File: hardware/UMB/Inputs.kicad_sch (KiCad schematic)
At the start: 30 parts, among them J1 FTSH-107-01-L-D-K, J10 Conn_01x04, J11 Conn_01x04, J12 Conn_01x04, J13 Conn_01x04, J14 Conn_01x04, J15 Conn_01x04, J2 Conn_01x02, J3 Conn_01x02, J4 Conn_01x03, J5 Conn_01x03, J6 Conn_01x03, J7 Conn_01x03, J8 Conn_01x03, J9 Conn_01x03

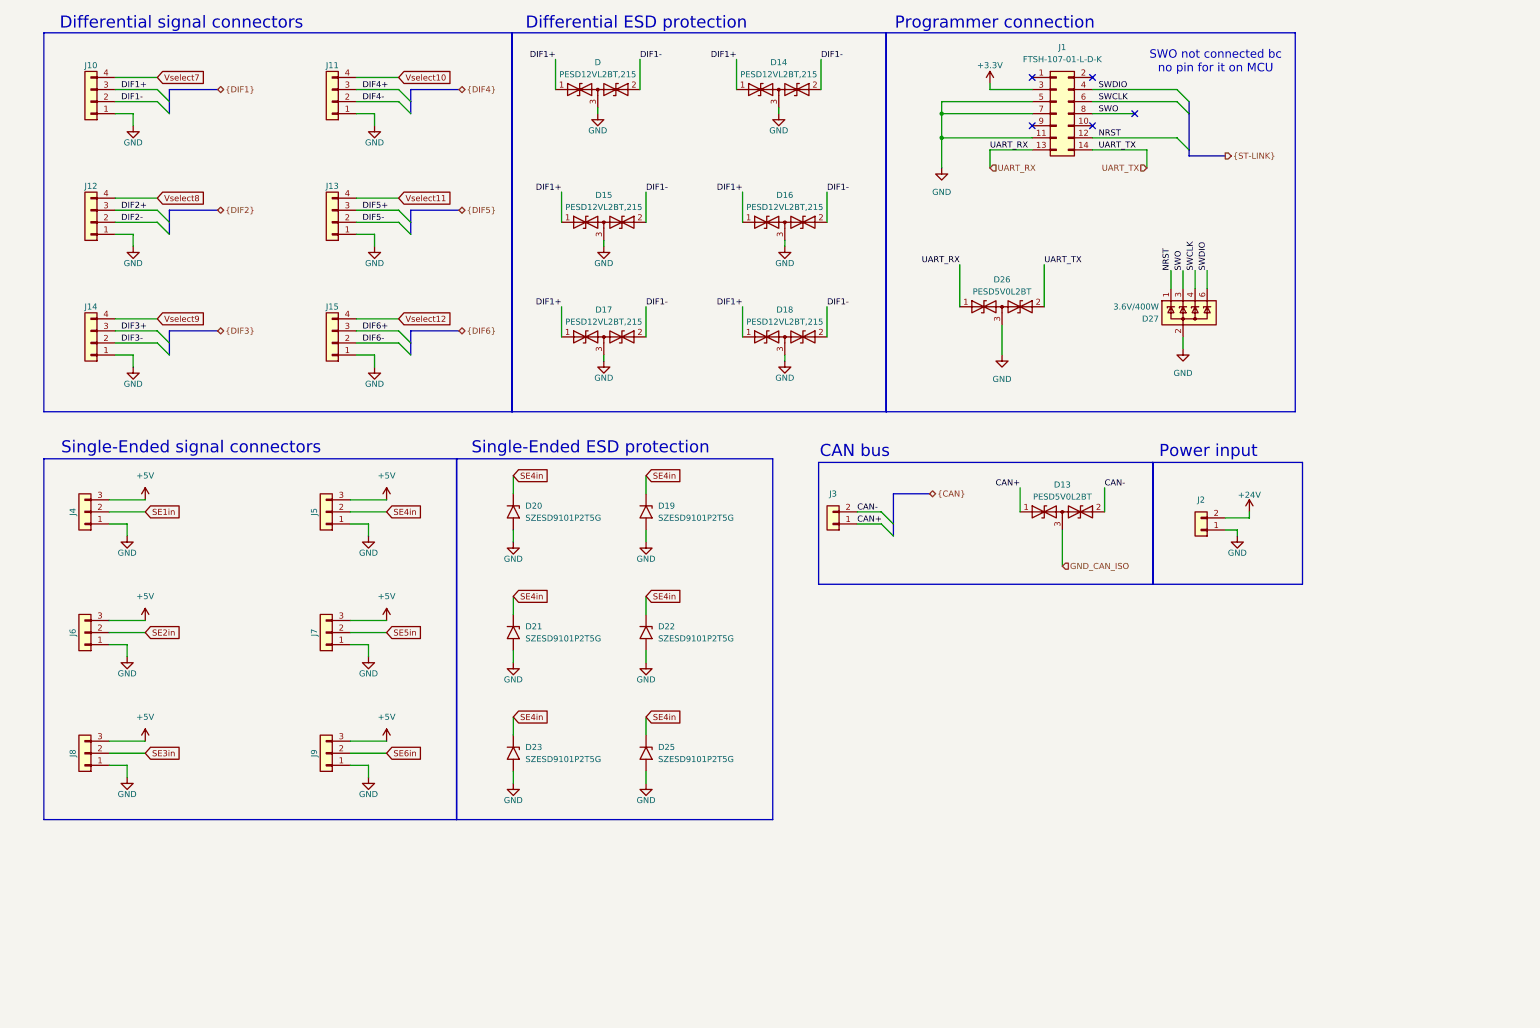
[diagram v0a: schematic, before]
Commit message: Power section done
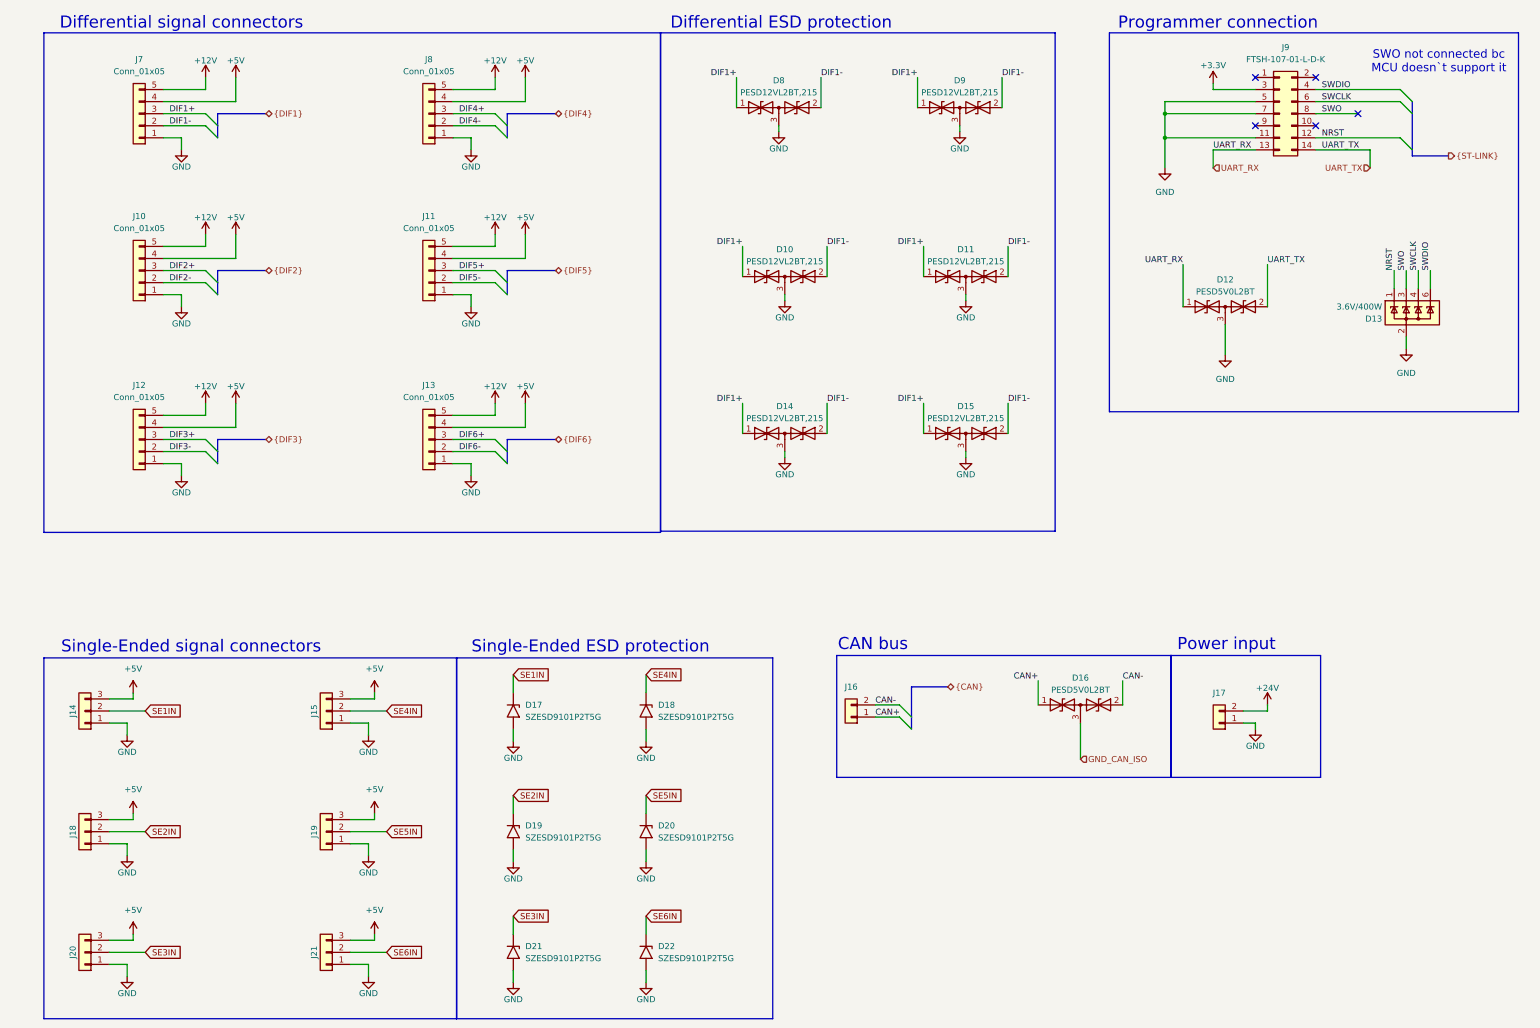
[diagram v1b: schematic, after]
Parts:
- removed J10, J11, J12, J13, J14, J15: Conn_01x04, symbol Connector_Generic:Conn_01x04
- added J10, J11, J12, J13, J7, J8: Conn_01x05, symbol Connector_Generic:Conn_01x05
- renumbered D15 to D10, D16 to D11, D26 to D12, D27 to D13, D17 to D14, D18 to D15, D13 to D16, D20 to D17, D19 to D18, D21 to D19, D22 to D20, D23 to D21, D25 to D22, D to D8, D14 to D9, J4 to J14, J5 to J15, J3 to J16, J2 to J17, J6 to J18, J7 to J19, J8 to J20, J9 to J21, J1 to J9
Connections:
- net +5V: now also J10.4 (Pin_4), J11.4 (Pin_4), J12.4 (Pin_4), J13.4 (Pin_4), J7.4 (Pin_4), J8.4 (Pin_4)
- net DIF1+: now also J7.3 (Pin_3)
- net DIF1-: now also J7.2 (Pin_2)
- net DIF2+: now also J10.3 (Pin_3)
- net DIF2-: now also J10.2 (Pin_2)
- net DIF3+: now also J12.3 (Pin_3)
- net DIF3-: now also J12.2 (Pin_2)
- net DIF4+: now also J8.3 (Pin_3)
- net DIF4-: now also J8.2 (Pin_2)
- net DIF5+: now also J11.3 (Pin_3)
- net DIF5-: now also J11.2 (Pin_2)
- net DIF6+: now also J13.3 (Pin_3)
- net DIF6-: now also J13.2 (Pin_2)
- net GND: now also J10.1 (Pin_1), J11.1 (Pin_1), J12.1 (Pin_1), J13.1 (Pin_1), J7.1 (Pin_1), J8.1 (Pin_1)
- net SE1in renamed SE1IN
- net SE1IN: now also D17.1 (A1)
- net SE2in renamed SE2IN
- net SE2IN: now also D19.1 (A1)
- net SE3in renamed SE3IN
- net SE3IN: now also D21.1 (A1)
- removed net SE4in: D17.1 (A1), D18.1 (A1), D19.1 (A1), D20.1 (A1), D21.1 (A1), D22.1 (A1), J15.2 (Pin_2)
- net SE5in renamed SE5IN
- net SE5IN: now also D20.1 (A1)
- net SE6in renamed SE6IN
- net SE6IN: now also D22.1 (A1)
- new net +12V: J10.5 (Pin_5), J11.5 (Pin_5), J12.5 (Pin_5), J13.5 (Pin_5), J7.5 (Pin_5), J8.5 (Pin_5)
- new net SE4IN: D18.1 (A1), J15.2 (Pin_2)
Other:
- note added: "SWO not connected bc MCU doesn`t support it"
- note removed: "SWO not connected bc no pin for it on MCU"
- moved on the sheet: D10, D11, D12, D13, D14, D15, D16, D17, D18, D19, D20, D21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
